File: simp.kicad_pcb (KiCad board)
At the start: 2 copper layers, 80 x 100 mm, 59 parts, among them J1 AVR-ISP-6, J2 I2C, J3 USB_C_Receptacle_USB2.0, SW1 MX_SW_solder, SW10 MX_SW_solder, SW11 MX_SW_solder, SW12 MX_SW_solder, SW13 MX_SW_solder, SW14 MX_SW_solder, SW15 MX_SW_solder, SW16 MX_SW_solder, SW2 MX_SW_solder, SW3 MX_SW_solder, SW4 MX_SW_solder, SW5 MX_SW_solder, SW6 MX_SW_solder, SW7 MX_SW_solder, SW8 MX_SW_solder, SW9 MX_SW_solder, U1 ATmega32U4-M, U2 USBLC6-2P6, Y1 16MHz

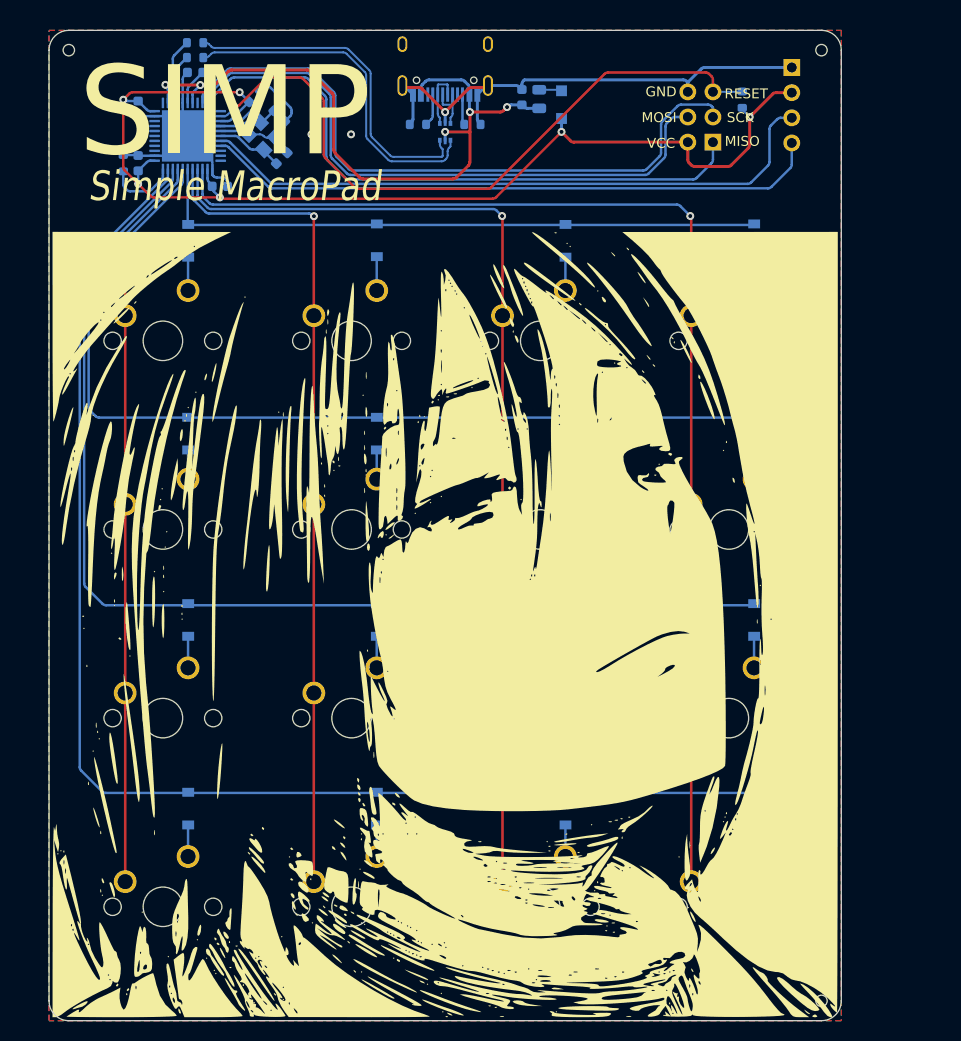
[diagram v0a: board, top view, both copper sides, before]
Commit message: version: bump version to 1.0.0
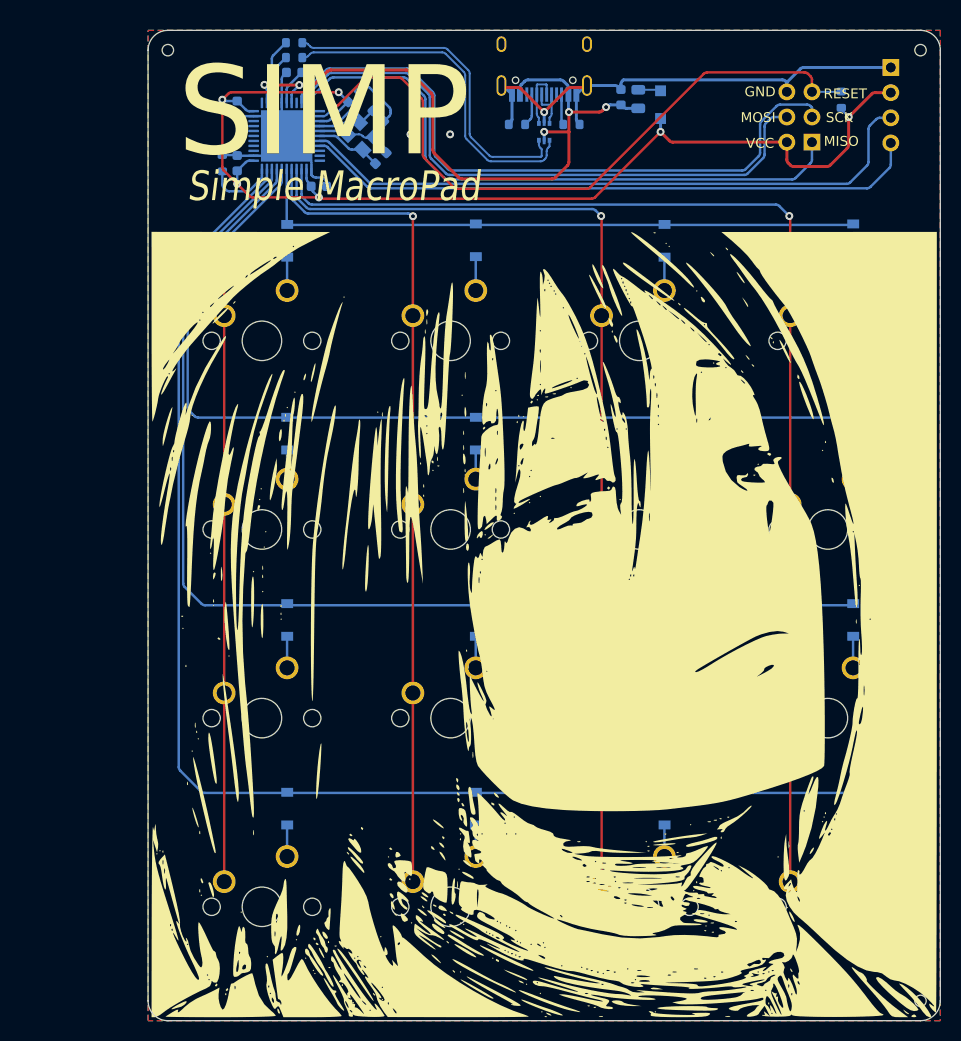
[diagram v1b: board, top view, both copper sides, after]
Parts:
- moved ? 10.0 mm to (108.0, 32.0)
- moved ? 10.0 mm to (32.0, 128.0)
- moved ? 10.0 mm to (108.0, 128.0)
- moved ? 10.0 mm to (32.0, 32.0)
- moved C1 10.0 mm to (44.8, 34.2)
- moved C2 10.0 mm to (53.5, 42.9)
- moved C3 10.0 mm to (53.2, 38.7)
- moved C4 10.0 mm to (39.0, 37.9)
- moved C5 10.0 mm to (50.8, 36.7)
- moved C6 10.0 mm to (39.0, 43.4)
- moved C7 10.0 mm to (47.2, 45.8)
- moved C8 10.0 mm to (77.8, 36.8)
- moved D1 10.0 mm to (44.1, 51.2)
- moved D10 10.0 mm to (63.1, 89.5)
- moved D11 10.0 mm to (82.2, 89.5)
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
